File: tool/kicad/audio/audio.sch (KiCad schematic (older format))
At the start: 28 parts, among them K2 CONN_3, P1 CONN_6, P5 MIDI-IN, U5 LM386, U6 LM386, U7 ACPL-M21L

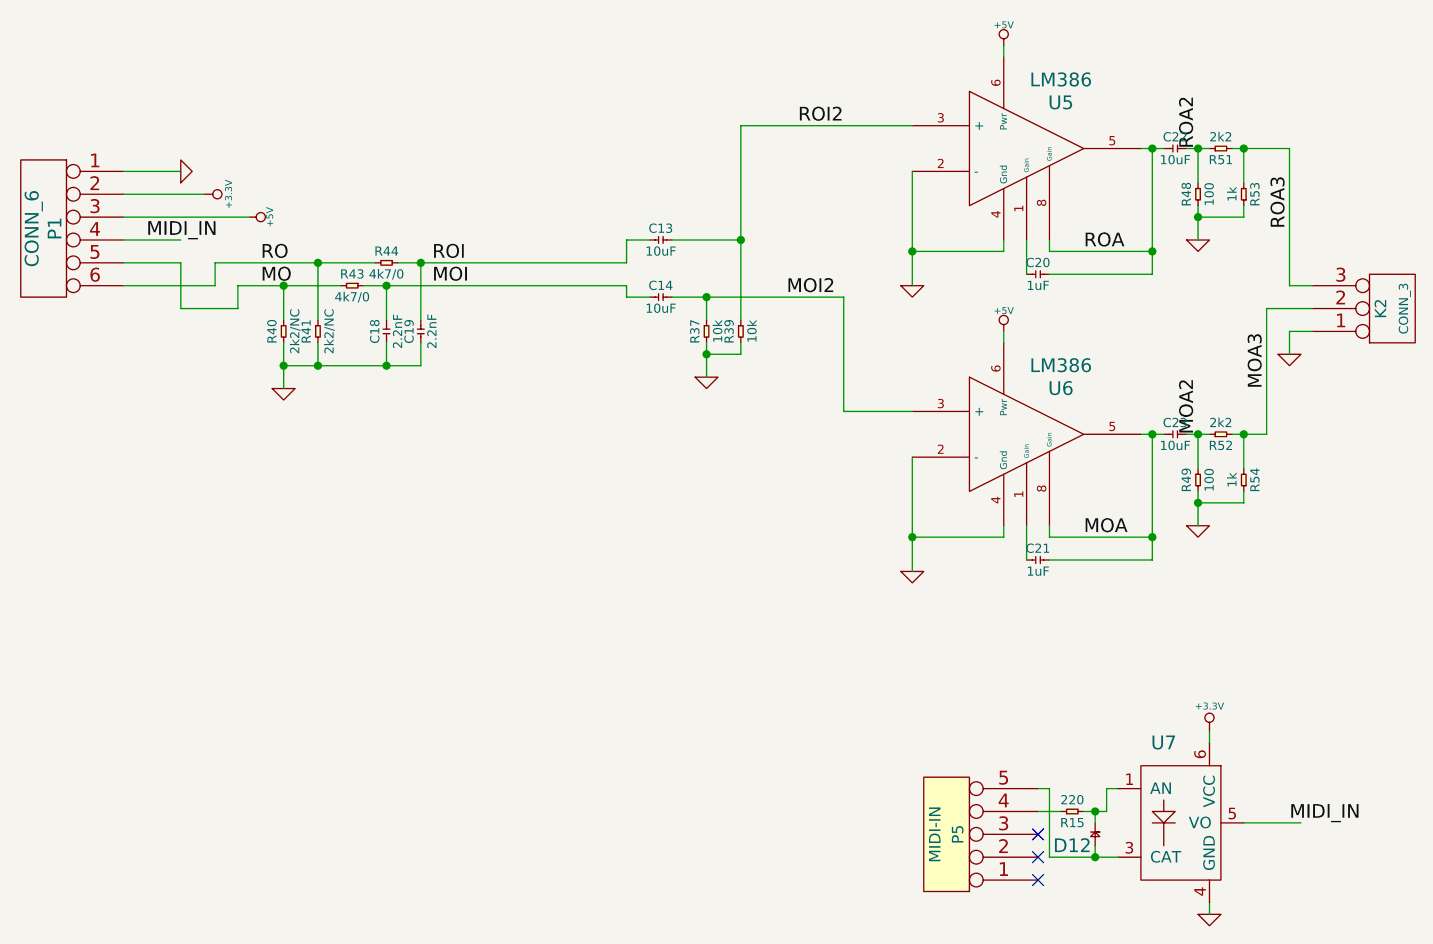
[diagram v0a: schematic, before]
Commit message: layout
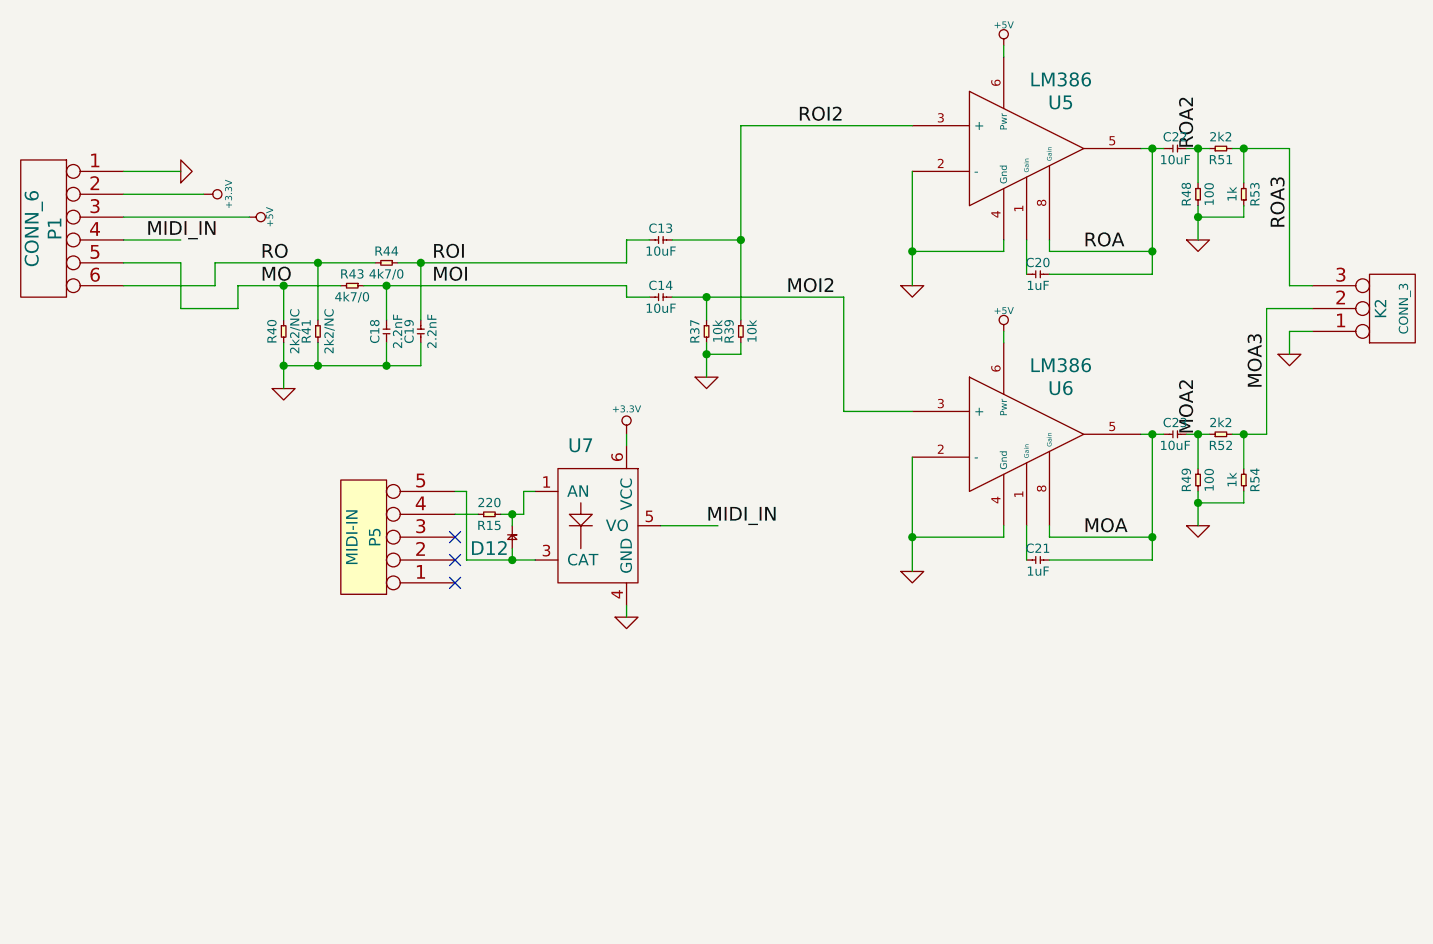
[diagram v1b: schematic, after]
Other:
- moved on the sheet: D12, P5, R15, U7
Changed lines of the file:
@@
 L CONN_5 P5
 U 1 1 52F74BDD
-P 5500 4500
-F 0 "P5" V 5450 4500 50  0000 C CNN
-F 1 "MIDI-IN" V 5550 4500 50  0000 C CNN
-F 2 "" H 5500 4500 60  0000 C CNN
-F 3 "" H 5500 4500 60  0000 C CNN
-	1    5500 4500
+P 2950 3200
+F 0 "P5" V 2900 3200 50  0000 C CNN
+F 1 "MIDI-IN" V 3000 3200 50  0000 C CNN
+F 2 "" H 2950 3200 60  0000 C CNN
+F 3 "" H 2950 3200 60  0000 C CNN
+	1    2950 3200
 	-1   0    0    1
 $EndComp
@@
 L R R15
 U 1 1 52F74BF4
-P 6050 4400
-F 0 "R15" H 6050 4450 40  0000 C CNN
-F 1 "220" H 6050 4350 40  0000 C CNN
-F 2 "" H 6050 4400 60  0000 C CNN
-F 3 "" H 6050 4400 60  0000 C CNN
-	1    6050 4400
+P 3500 3100
+F 0 "R15" H 3500 3150 40  0000 C CNN
+F 1 "220" H 3500 3050 40  0000 C CNN
+F 2 "" H 3500 3100 60  0000 C CNN
+F 3 "" H 3500 3100 60  0000 C CNN
+	1    3500 3100
 	-1   0    0    1
 $EndComp
@@
 Connection ~ 4450 2150
 Wire Wire Line
-	6100 4400 6200 4400
-Wire Wire Line
-	5900 4400 6000 4400
-Wire Wire Line
-	5950 4600 6250 4600
-Wire Wire Line
-	5950 4600 5950 4300
-Wire Wire Line
-	5950 4300 5900 4300
-Text Label 7000 4450 0    60   ~ 0
+	3550 3100 3650 3100
+Wire Wire Line
+	3350 3100 3450 3100
+Wire Wire Line
+	3400 3300 3700 3300
+Wire Wire Line
+	3400 3300 3400 3000
+Wire Wire Line
+	3400 3000 3350 3000
+Text Label 4450 3150 0    60   ~ 0
 MIDI_IN
 $Comp
 L D D12
 U 1 1 52F758D1
-P 6150 4500
-F 0 "D12" V 6100 4600 60  0000 C CNN
-F 1 "D" H 6155 4435 60  0001 C CNN
-F 2 "" H 6150 4500 60  0000 C CNN
-F 3 "" H 6150 4500 60  0000 C CNN
-	1    6150 4500
+P 3600 3200
+F 0 "D12" V 3550 3300 60  0000 C CNN
+F 1 "D" H 3605 3135 60  0001 C CNN
+F 2 "" H 3600 3200 60  0000 C CNN
+F 3 "" H 3600 3200 60  0000 C CNN
+	1    3600 3200
 	0    -1   -1   0
 $EndComp
 Wire Wire Line
-	6150 4400 6150 4450
-Connection ~ 6150 4400
-Wire Wire Line
-	6150 4550 6150 4600
-Connection ~ 6150 4600
+	3600 3100 3600 3150
+Connection ~ 3600 3100
+Wire Wire Line
+	3600 3250 3600 3300
+Connection ~ 3600 3300
 $Comp
 L CONN_3 K2
@@
 L ACPL-M21L U7
 U 1 1 52F8C674
-P 6650 4500
-F 0 "U7" H 6450 4900 60  0000 C CNN
-F 1 "ACPL-M21L" H 6300 4250 60  0001 C CNN
-F 2 "" H 6650 4500 60  0000 C CNN
-F 3 "" H 6650 4500 60  0000 C CNN
-	1    6650 4500
-	1    0    0    -1
-$EndComp
-Wire Wire Line
-	6250 4300 6200 4300
-Wire Wire Line
-	6200 4300 6200 4400
+P 4100 3200
+F 0 "U7" H 3900 3600 60  0000 C CNN
+F 1 "ACPL-M21L" H 3750 2950 60  0001 C CNN
+F 2 "" H 4100 3200 60  0000 C CNN
+F 3 "" H 4100 3200 60  0000 C CNN
+	1    4100 3200
+	1    0    0    -1
+$EndComp
+Wire Wire Line
+	3700 3000 3650 3000
+Wire Wire Line
+	3650 3000 3650 3100
 $Comp
 L GND #PWR010
 U 1 1 52F8C9F7
-P 6650 4850
-F 0 "#PWR010" H 6650 4850 30  0001 C CNN
-F 1 "GND" H 6650 4780 30  0001 C CNN
-F 2 "" H 6650 4850 60  0000 C CNN
-F 3 "" H 6650 4850 60  0000 C CNN
-	1    6650 4850
-	1    0    0    -1
-$EndComp
-Wire Wire Line
-	6650 4800 6650 4850
+P 4100 3550
+F 0 "#PWR010" H 4100 3550 30  0001 C CNN
+F 1 "GND" H 4100 3480 30  0001 C CNN
+F 2 "" H 4100 3550 60  0000 C CNN
+F 3 "" H 4100 3550 60  0000 C CNN
+	1    4100 3550
+	1    0    0    -1
+$EndComp
+Wire Wire Line
+	4100 3500 4100 3550
 $Comp
 L +3.3V #PWR011
 U 1 1 52F8CBAF
-P 6650 4050
-F 0 "#PWR011" H 6650 4010 30  0001 C CNN
-F 1 "+3.3V" H 6650 4160 30  0000 C CNN
-F 2 "" H 6650 4050 60  0000 C CNN
-F 3 "" H 6650 4050 60  0000 C CNN
-	1    6650 4050
-	1    0    0    -1
-$EndComp
-Wire Wire Line
-	6650 4050 6650 4100
-Wire Wire Line
-	7050 4450 6800 4450
-NoConn ~ 5900 4500
-NoConn ~ 5900 4600
-NoConn ~ 5900 4700
+P 4100 2750
+F 0 "#PWR011" H 4100 2710 30  0001 C CNN
+F 1 "+3.3V" H 4100 2860 30  0000 C CNN
+F 2 "" H 4100 2750 60  0000 C CNN
+F 3 "" H 4100 2750 60  0000 C CNN
+	1    4100 2750
+	1    0    0    -1
+$EndComp
+Wire Wire Line
+	4100 2750 4100 2800
+Wire Wire Line
+	4500 3150 4250 3150
+NoConn ~ 3350 3200
+NoConn ~ 3350 3300
+NoConn ~ 3350 3400
 Wire Wire Line
 	4100 2000 4100 1900
